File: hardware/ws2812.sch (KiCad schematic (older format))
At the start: 0 parts

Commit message: update,
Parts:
- added D?: WS2812, LED_SMD:LED_WS2812_PLCC6_5.0x5.0mm_P1.6mm, symbol LED:WS2812

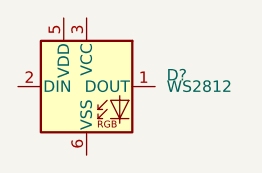
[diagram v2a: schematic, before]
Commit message: update,
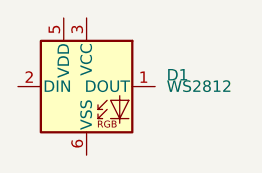
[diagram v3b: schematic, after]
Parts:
- gave numbers to parts that had none: 1
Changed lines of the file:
@@
 EESchema Schematic File Version 4
 LIBS:eval_board-cache
-LIBS:bb-ch340t-cache
 EELAYER 29 0
 EELAYER END
 $Descr A4 11693 8268
 encoding utf-8
-Sheet 8 20
+Sheet 8 22
 Title ""
 Date ""
@@
 $EndBitmap
 $Comp
-L LED:WS2812 D?
+L LED:WS2812 D1
 U 1 1 5CE91B05
 P 3650 3050
-F 0 "D?" H 4000 3100 50  0000 L CNN
+F 0 "D1" H 4000 3100 50  0000 L CNN
 F 1 "WS2812" H 4000 3050 50  0000 L CNN
 F 2 "LED_SMD:LED_WS2812_PLCC6_5.0x5.0mm_P1.6mm" H 3700 2750 50  0001 L TNN

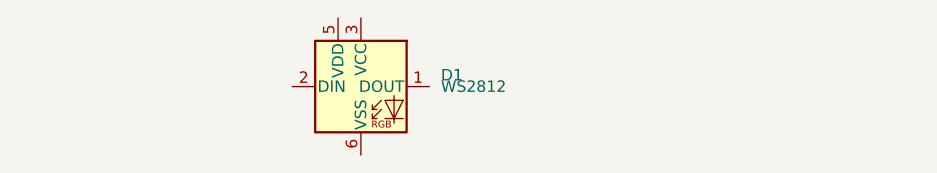
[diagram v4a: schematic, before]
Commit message: update,
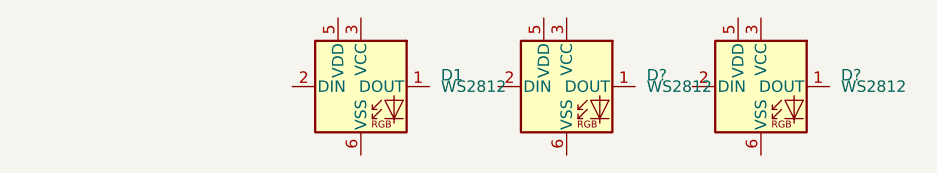
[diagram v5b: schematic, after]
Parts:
- added D? (x2): WS2812, LED_SMD:LED_WS2812_PLCC6_5.0x5.0mm_P1.6mm, symbol LED:WS2812
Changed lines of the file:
@@
 $Descr A4 11693 8268
 encoding utf-8
-Sheet 8 21
+Sheet 6 20
 Title ""
 Date ""
@@
 	1    0    0    -1
 $EndComp
+$Comp
+L LED:WS2812 D?
+U 1 1 5CF2390D
+P 4550 3050
+F 0 "D?" H 4900 3100 50  0000 L CNN
+F 1 "WS2812" H 4900 3050 50  0000 L CNN
+F 2 "LED_SMD:LED_WS2812_PLCC6_5.0x5.0mm_P1.6mm" H 4600 2750 50  0001 L TNN
+F 3 "https://cdn-shop.adafruit.com/datasheets/WS2812.pdf" H 4650 2675 50  0001 L TNN
+	1    4550 3050
+	1    0    0    -1
+$EndComp
+$Comp
+L LED:WS2812 D?
+U 1 1 5CF23CE3
+P 5400 3050
+F 0 "D?" H 5750 3100 50  0000 L CNN
+F 1 "WS2812" H 5750 3050 50  0000 L CNN
+F 2 "LED_SMD:LED_WS2812_PLCC6_5.0x5.0mm_P1.6mm" H 5450 2750 50  0001 L TNN
+F 3 "https://cdn-shop.adafruit.com/datasheets/WS2812.pdf" H 5500 2675 50  0001 L TNN
+	1    5400 3050
+	1    0    0    -1
+$EndComp

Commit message: update,
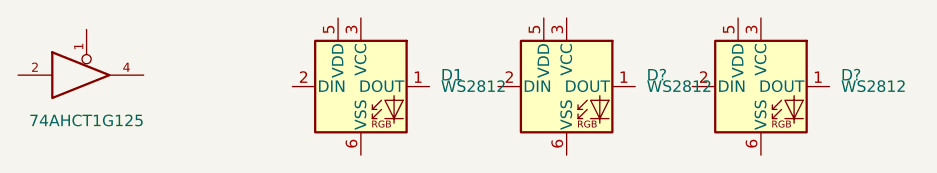
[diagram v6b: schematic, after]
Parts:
- added U?: 74AHCT1G125, Package_TO_SOT_SMD:SOT-23-5_HandSoldering, symbol 74xGxx:74AHCT1G125
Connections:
- new net GND: U?.3 (GND)
- new net VCC: U?.5 (VCC)
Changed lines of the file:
@@
+	1    0    0    -1
+$EndComp
+$Comp
+L 74xGxx:74AHCT1G125 U?
+U 1 1 5CFAEDA6
+P 2450 3000
+F 0 "U?" H 2450 2750 50  0001 C CNN
+F 1 "74AHCT1G125" H 2450 2800 50  0000 C CNN
+F 2 "Package_TO_SOT_SMD:SOT-23-5_HandSoldering" H 2450 3000 50  0001 C CNN
+F 3 "http://www.ti.com/lit/sg/scyt129e/scyt129e.pdf" H 2450 3000 50  0001 C CNN
+	1    2450 3000
 	1    0    0    -1
 $EndComp

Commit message: update,
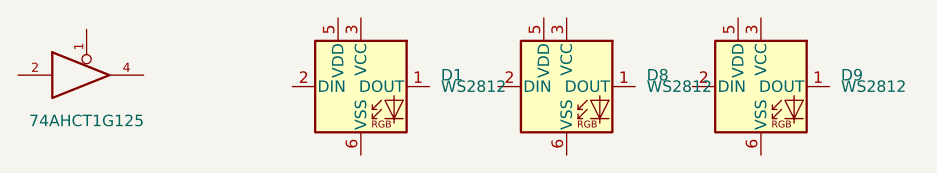
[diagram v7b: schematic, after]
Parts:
- gave numbers to parts that had none: 3
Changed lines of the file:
@@
 $EndComp
 $Comp
-L LED:WS2812 D?
+L LED:WS2812 D8
 U 1 1 5CF2390D
 P 4550 3050
-F 0 "D?" H 4900 3100 50  0000 L CNN
+F 0 "D8" H 4900 3100 50  0000 L CNN
 F 1 "WS2812" H 4900 3050 50  0000 L CNN
 F 2 "LED_SMD:LED_WS2812_PLCC6_5.0x5.0mm_P1.6mm" H 4600 2750 50  0001 L TNN
@@
 $EndComp
 $Comp
-L LED:WS2812 D?
+L LED:WS2812 D9
 U 1 1 5CF23CE3
 P 5400 3050
-F 0 "D?" H 5750 3100 50  0000 L CNN
+F 0 "D9" H 5750 3100 50  0000 L CNN
 F 1 "WS2812" H 5750 3050 50  0000 L CNN
 F 2 "LED_SMD:LED_WS2812_PLCC6_5.0x5.0mm_P1.6mm" H 5450 2750 50  0001 L TNN
@@
 $EndComp
 $Comp
-L 74xGxx:74AHCT1G125 U?
+L 74xGxx:74AHCT1G125 U7
 U 1 1 5CFAEDA6
 P 2450 3000
-F 0 "U?" H 2450 2750 50  0001 C CNN
+F 0 "U7" H 2450 2750 50  0001 C CNN
 F 1 "74AHCT1G125" H 2450 2800 50  0000 C CNN
 F 2 "Package_TO_SOT_SMD:SOT-23-5_HandSoldering" H 2450 3000 50  0001 C CNN
